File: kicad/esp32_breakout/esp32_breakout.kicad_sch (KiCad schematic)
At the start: 30 parts, among them J1 JST PH F, J10 JST PH F, J11 JST PH F, J2 JST PH F, J3 JST PH F, J4 DC-005 5.5x2.1mm, J5 Deans T-Plug M, J6 Header F, J7 Header F, J8 Header F, J9 JST PH F, Q1 BSS123, SW1 SS12D10, U1 ESP32 DEV KIT 30-pin, U2 Mini560-Pro

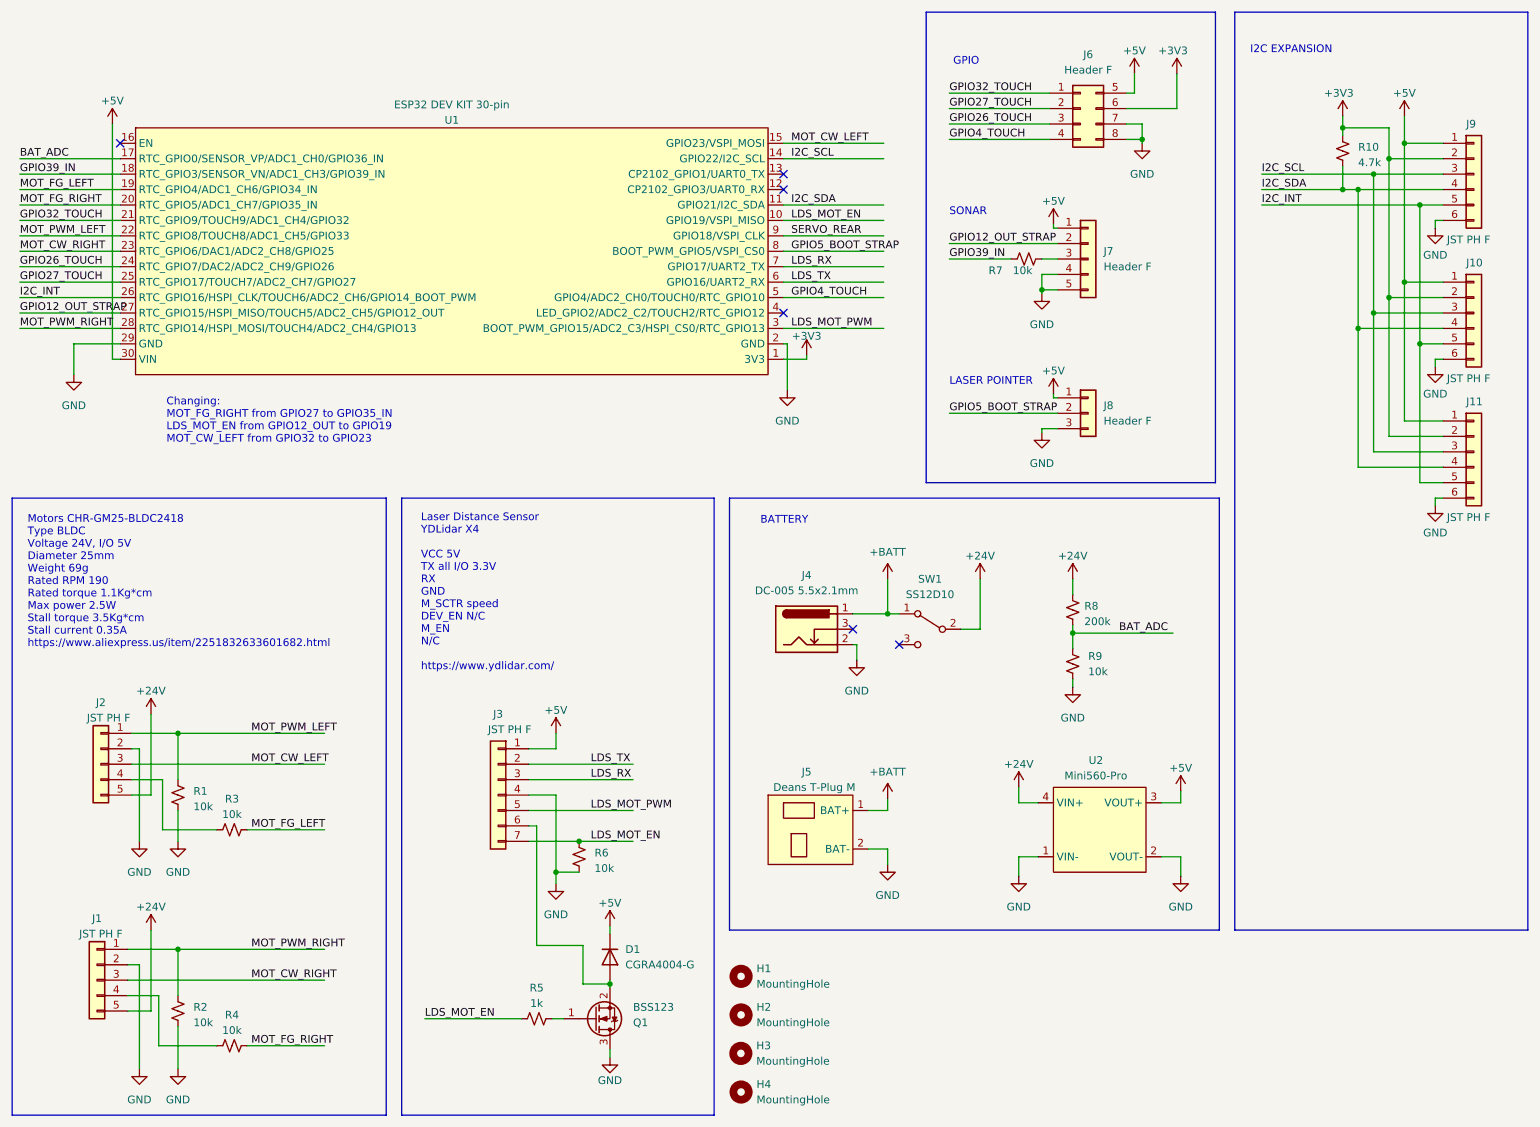
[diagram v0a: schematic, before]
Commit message: PCB updated to product
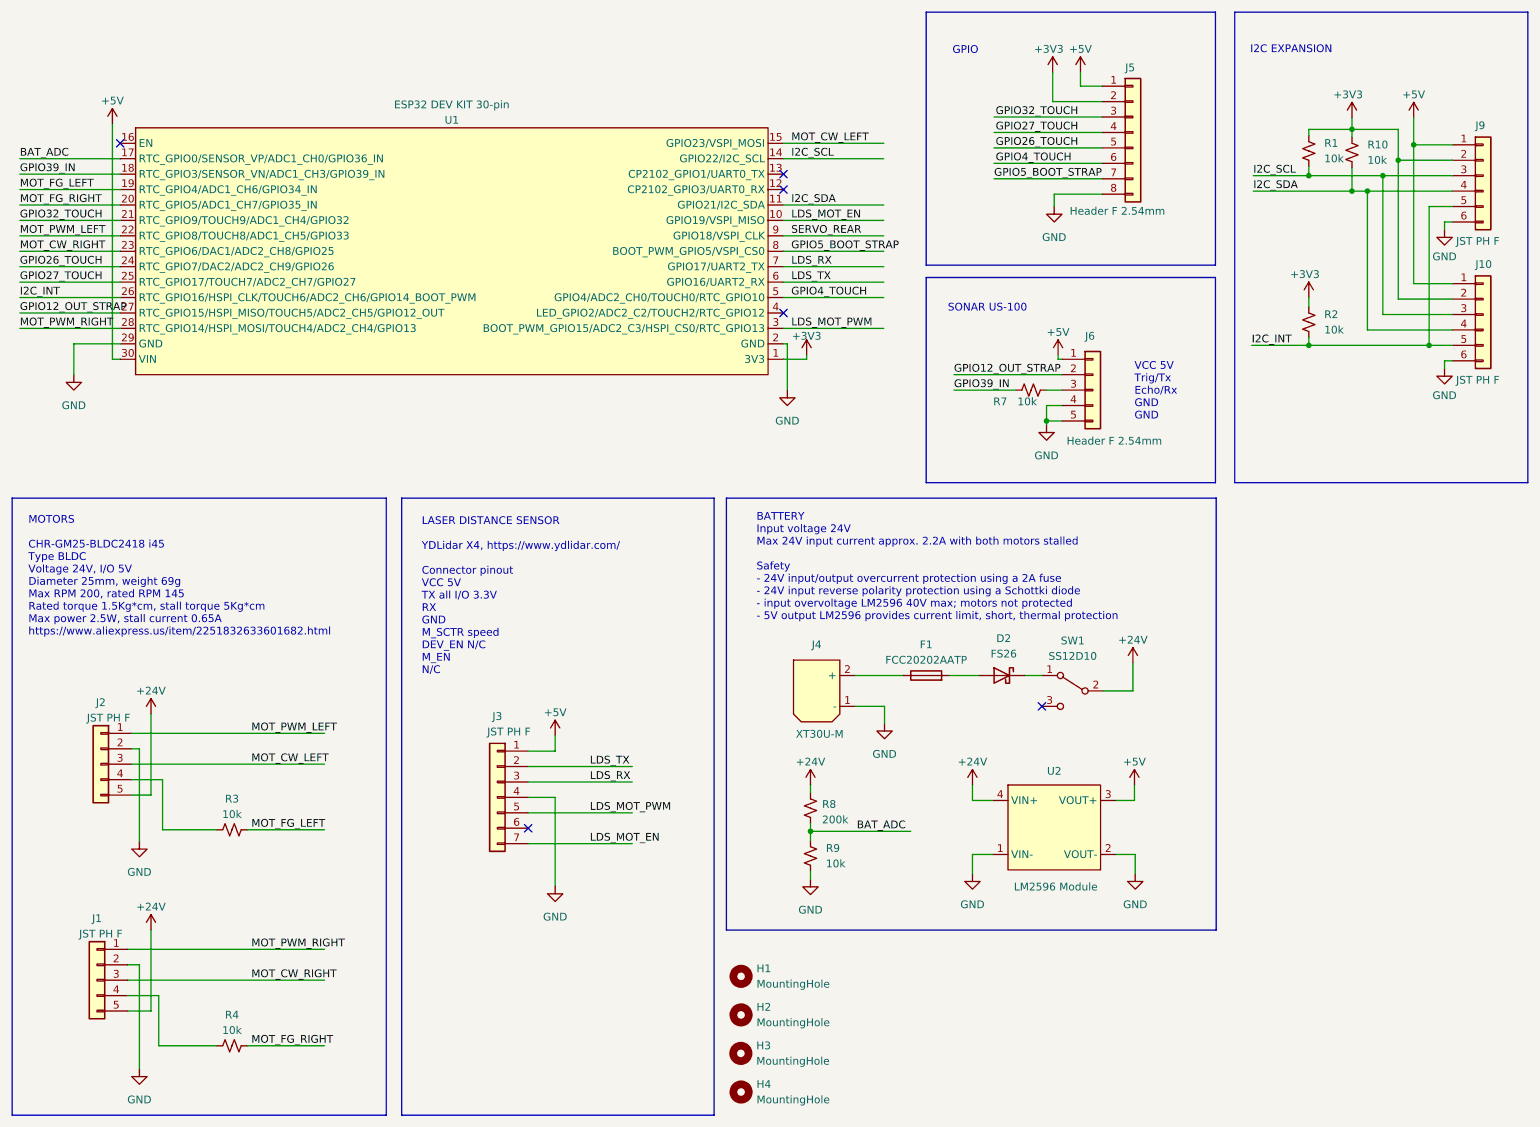
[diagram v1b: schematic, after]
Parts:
- removed D1: CGRA4004-G, Diode_SMD:D_SMA, symbol Device:D
- removed J11: JST PH F, Connector_JST:JST_PH_B6B-PH-K_1x06_P2.00mm_Vertical, symbol Connector_Generic:Conn_01x06
- removed J4: DC-005 5.5x2.1mm, Connector_BarrelJack:BarrelJack_GCT_DCJ200-10-A_Horizontal, symbol Connector:Barrel_Jack_Switch
- removed J5: Deans T-Plug M, Makerspet:DEANS-T-PLUG, symbol Makerspet:Deans T-Plug
- removed J6: Header F, Connector_PinHeader_2.54mm:PinHeader_2x04_P2.54mm_Vertical, symbol Connector_Generic:Conn_02x04_Top_Bottom
- removed J8: Header F, Connector_PinHeader_2.54mm:PinHeader_1x03_P2.54mm_Vertical, symbol Connector_Generic:Conn_01x03
- removed Q1: BSS123, Package_TO_SOT_SMD:SOT-23, symbol Transistor_FET:BSS123
- removed R5: 1k, Resistor_SMD:R_0603_1608Metric, symbol Device:R_Small_US
- removed R6: 10k, Resistor_SMD:R_0603_1608Metric, symbol Device:R_Small_US
- removed U2: Mini560-Pro, Makerspet:Mini560-Pro, symbol Makerspet:DC-DC
- added D2: FS26, Diode_SMD:D_SOD-123F, symbol Device:D_Schottky
- added F1: FCC20202AATP, Fuse:Fuse_0805_2012Metric, symbol Device:Fuse
- added J4: XT30U-M, Connector_AMASS:AMASS_XT30U-M_1x02_P5.0mm_Vertical, symbol Makerspet:XT30UPB-M
- added J5: Header F 2.54mm, Connector_PinHeader_2.54mm:PinHeader_1x08_P2.54mm_Vertical, symbol Connector_Generic:Conn_01x08
- added U2: LM2596 Module, Makerspet:LM2596 Module, symbol Makerspet:DC-DC Module
- J6: renamed from J7; value Header F -> Header F 2.54mm
- R10: value 4.7k -> 10k
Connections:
- net +24V: now also U2.4 (VIN+)
- net +3V3: now also R1.1, R2.1, J5.2 (Pin_2)
- net +5V: now also J5.1 (Pin_1), U2.3 (VOUT+)
- net GND: now also J4.1 (-), J5.8 (Pin_8), U2.1 (VIN-), U2.2 (VOUT-); no longer R1.2, R2.2
- net GPIO26_TOUCH: now also J5.5 (Pin_5)
- net GPIO27_TOUCH: now also J5.4 (Pin_4)
- net GPIO32_TOUCH: now also J5.3 (Pin_3)
- net GPIO4_TOUCH: now also J5.6 (Pin_6)
- net GPIO5_BOOT_STRAP: now also J5.7 (Pin_7)
- net I2C_INT: now also R2.2
- net I2C_SCL: now also R1.2
- net MOT_PWM_LEFT: no longer R1.1
- net MOT_PWM_RIGHT: no longer R2.1
- net +BATT: no longer names the net of SW1.1 (A)
- net +BATT: now also D2.1 (K)
- new net: F1.1, J4.2 (+)
- new net: D2.2 (A), F1.2
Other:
- note added: "BATTERY Input voltage 24V Max 24V input current approx. 2.2A with both motors stalled Safety - 24V input/output overcurrent protection using a 2A fuse - 24V input reverse polarity protection using a Schottki diode - input overvoltage LM2596 40V max; motors not protected - 5V output LM2596 provides current limit, short, thermal protection"
- note added: "LASER DISTANCE SENSOR YDLidar X4, https://www.ydlidar.com/ Connector pinout VCC 5V TX all I/O 3.3V RX GND M_SCTR speed DEV_EN N/C M_EN N/C"
- note added: "MOTORS CHR-GM25-BLDC2418 i45 Type BLDC Voltage 24V, I/O 5V Diameter 25mm, weight 69g Max RPM 200, rated RPM 145 Rated torque 1.5Kg*cm, stall torque 5Kg*cm Max power 2.5W, stall current 0.65A https://www.aliexpress.us/item/2251832633601682.html"
- note added: "SONAR US-100"
- note added: "VCC 5V Trig/Tx Echo/Rx GND GND"
- note removed: "BATTERY"
- note removed: "Changing: MOT_FG_RIGHT from GPIO27 to GPIO35_IN LDS_MOT_EN from GPIO12_OUT to GPIO19 MOT_CW_LEFT from GPIO32 to GPIO23"
- note removed: "LASER POINTER"
- note removed: "Laser Distance Sensor YDLidar X4 VCC 5V TX all I/O 3.3V RX GND M_SCTR speed DEV_EN N/C M_EN N/C https://www.ydlidar.com/"
- note removed: "Motors CHR-GM25-BLDC2418 Type BLDC Voltage 24V, I/O 5V Diameter 25mm Weight 69g Rated RPM 190 Rated torque 1.1Kg*cm Max power 2.5W Stall torque 3.5Kg*cm Stall current 0.35A https://www.aliexpress.us/item/2251832633601682.html"
- note removed: "SONAR"
- moved on the sheet: J10, J6, J9, R10, R7, R8, R9, SW1
